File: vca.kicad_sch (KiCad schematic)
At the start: 13 parts, among them U1 LM301, U2 LM301, U3 LM301, U4 LM1496, U5 LM301

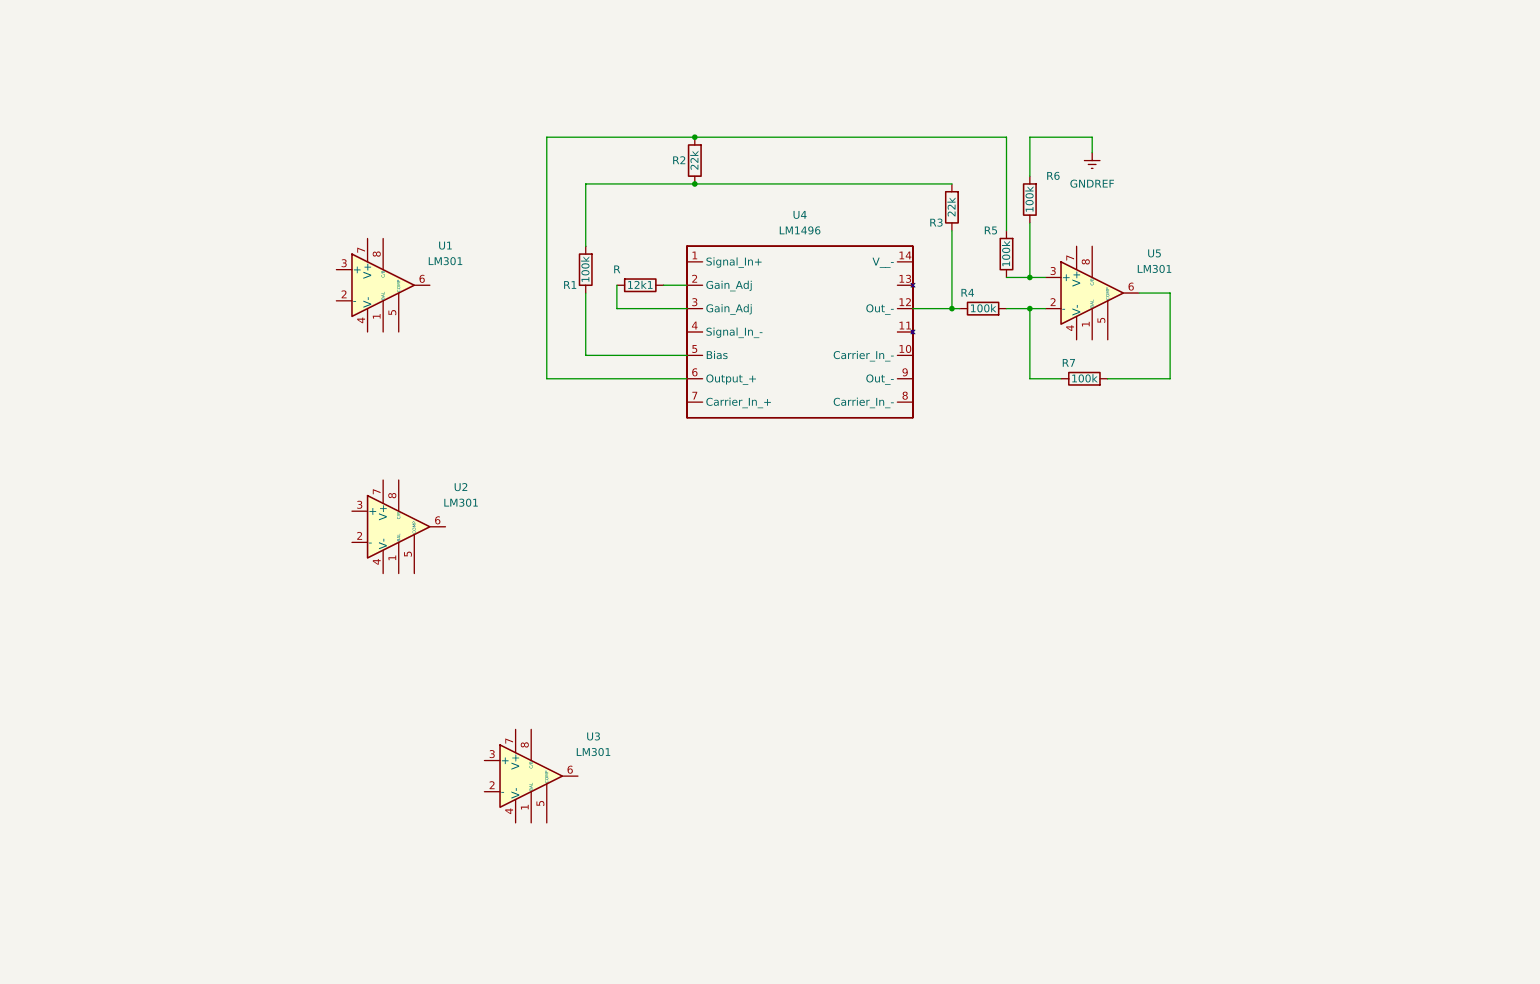
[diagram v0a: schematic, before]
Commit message: modificato:             operational.bak 	modificato:             operational.kicad_sym 	modificato:             vca.kicad_sch
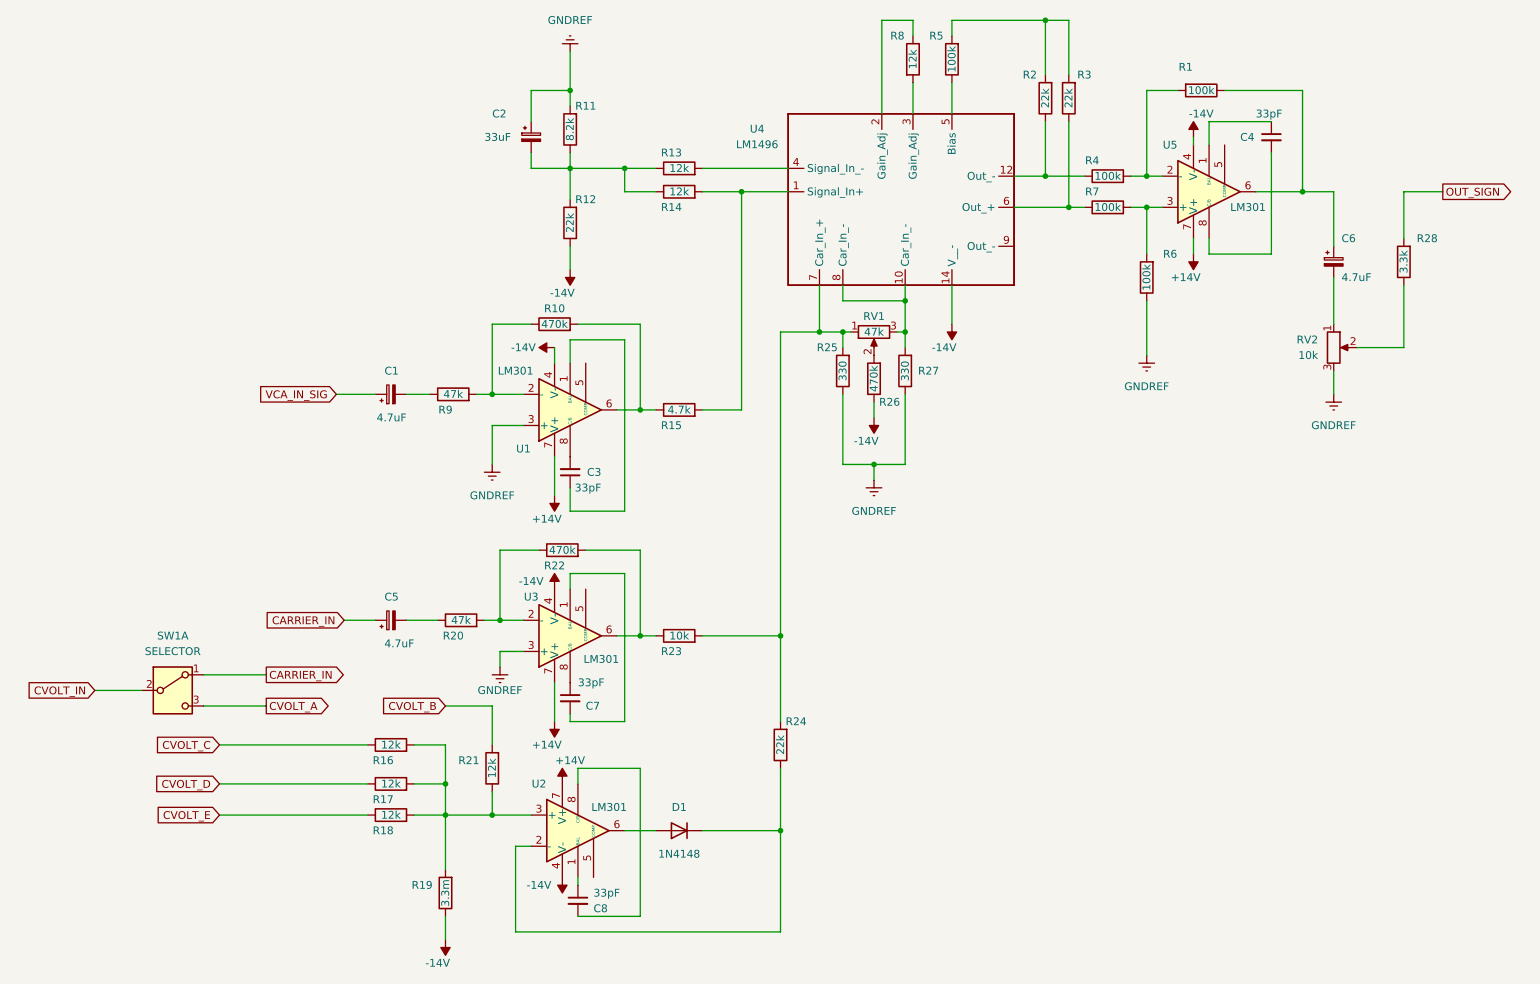
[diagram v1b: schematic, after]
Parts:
- added C1, C5, C6: 4.7uF, symbol Device:C_Polarized_Small
- added C2: 33uF, symbol Device:C_Polarized_Small
- added C3, C4, C7, C8: 33pF, symbol Device:C_Small
- added D1: 1N4148, Diode_THT:D_DO-35_SOD27_P7.62mm_Horizontal, symbol Diode:1N4148
- added R10, R22, R26: 470k, symbol Device:R
- added R11: 8.2k, symbol Device:R
- added R12, R24: 22k, symbol Device:R
- added R13, R14, R16, R17, R18, R21: 12k, symbol Device:R
- added R15: 4.7k, symbol Device:R
- added R19: 3.3m, symbol Device:R
- added R20, R9: 47k, symbol Device:R
- added R23: 10k, symbol Device:R
- added R25, R27: 330, symbol Device:R
- added R28: 3.3k, symbol Device:R
- added RV1: 47k, symbol Device:R_Potentiometer
- added RV2: 10k, symbol Device:R_Potentiometer
- added SW1: SELECTOR, symbol Switch:SW_DPDT_x2
- R8: renamed from 12k1; value R -> 12k
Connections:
- net GNDREF: now also R6.1, U1.3 (+), U3.3 (+), C2.1, R11.2, R25.1, R27.1, RV2.3; no longer R6.2
- net at R2.2, R5.2: now also R3.2; no longer U4.6 (Output_+)
- net at U5.1 (BAL): now also C4.1
- net at R4.2, U5.2 (-): now also R1.2; no longer R7.1
- net -14V: now reaches U5.4 (V-)
- net -14V: now also U1.4 (V-), U2.4 (V-), U3.4 (V-), U4.14 (V__-), R12.1, R19.1, R26.1
- net at R7.2: now also R6.2, U5.3 (+); no longer U5.6
- net +14V: now reaches U5.7 (V+)
- net +14V: now also U1.7 (V+), U2.7 (V+), U3.7 (V+)
- net at U5.8 (C/B): now also C4.2
- net at U3.1 (BAL): now also C7.2
- net at U3.2 (-): now also R20.2, R22.1
- net at U3.6: now also R22.2, R23.1
- net at U3.8 (C/B): now also C7.1
- net at R1.1: now also U5.6, C6.1; no longer U4.5 (Bias)
- net at U1.1 (BAL): now also C3.1
- net at U1.2 (-): now also R10.1, R9.2
- net at U1.6: now also R10.2, R15.1
- net at U1.8 (C/B): now also C3.2
- net at U2.1 (BAL): now also C8.1
- net at U2.2 (-): now also D1.1 (K), R24.1
- net at U2.3 (+): now also R16.2, R17.2, R18.2, R19.2, R21.1
- net at U2.6: now also D1.2 (A)
- net at U2.8 (C/B): now also C8.2
- net at R4.1, U4.12 (Out_-): now also R2.1; no longer R3.1
- net at U4.1 (Signal_In+): now also R14.2, R15.2
- net at U4.10 (Car_In_-): now also U4.8 (Car_In_-), R27.2, RV1.3
- net at U4.4 (Signal_In_-): now also R13.2
- net at U4.7 (Car_In_+): now also R23.2, R24.2, R25.2, RV1.1
- new net: C1.2, R9.1
- new net: R26.2, RV1.2
- new net: R5.1, U4.5 (Bias)
- new net: R3.1, R7.1, U4.6 (Out_+)
- new net: C5.2, R20.1
- new net: C2.2, R11.1, R12.2, R13.1, R14.1
- new net: C6.2, RV2.1
- new net: R28.1, RV2.2
- new net CARRIER_IN: C5.1, SW1.1 (A)
- new net CVOLT_A: SW1.3 (C)
- new net CVOLT_B: R21.2
- new net CVOLT_C: R16.1
- new net CVOLT_D: R17.1
- new net CVOLT_E: R18.1
- new net CVOLT_IN: SW1.2 (B)
- new net OUT_SIGN: R28.2
- new net VCA_IN_SIG: C1.1
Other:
- moved on the sheet: R1, R2, R3, R4, R5, R6, R7, R8, U1, U2, U3, U5
